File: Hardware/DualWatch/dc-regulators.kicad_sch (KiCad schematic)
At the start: 28 parts, among them Q1 IRLM2803, U16 SN74LV1T34DCK, U2 TPS63030DSK

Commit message: update pcb placing
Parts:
- C? (x2): footprint Capacitor_SMD:C_0402_1005Metric -> Capacitor_SMD:C_0603_1608Metric
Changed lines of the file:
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@@
       (effects (font (size 1.27 1.27)) (justify left))
     )
-    (property "Footprint" "Capacitor_SMD:C_0402_1005Metric" (at 129.2352 104.14 0)
+    (property "Footprint" "Capacitor_SMD:C_0603_1608Metric" (at 129.2352 104.14 0)
       (effects (font (size 1.27 1.27)) hide)
     )
@@
       (effects (font (size 1.27 1.27)) (justify left))
     )
-    (property "Footprint" "Capacitor_SMD:C_0402_1005Metric" (at 128.6002 52.07 0)
+    (property "Footprint" "Capacitor_SMD:C_0603_1608Metric" (at 128.6002 52.07 0)
       (effects (font (size 1.27 1.27)) hide)
     )

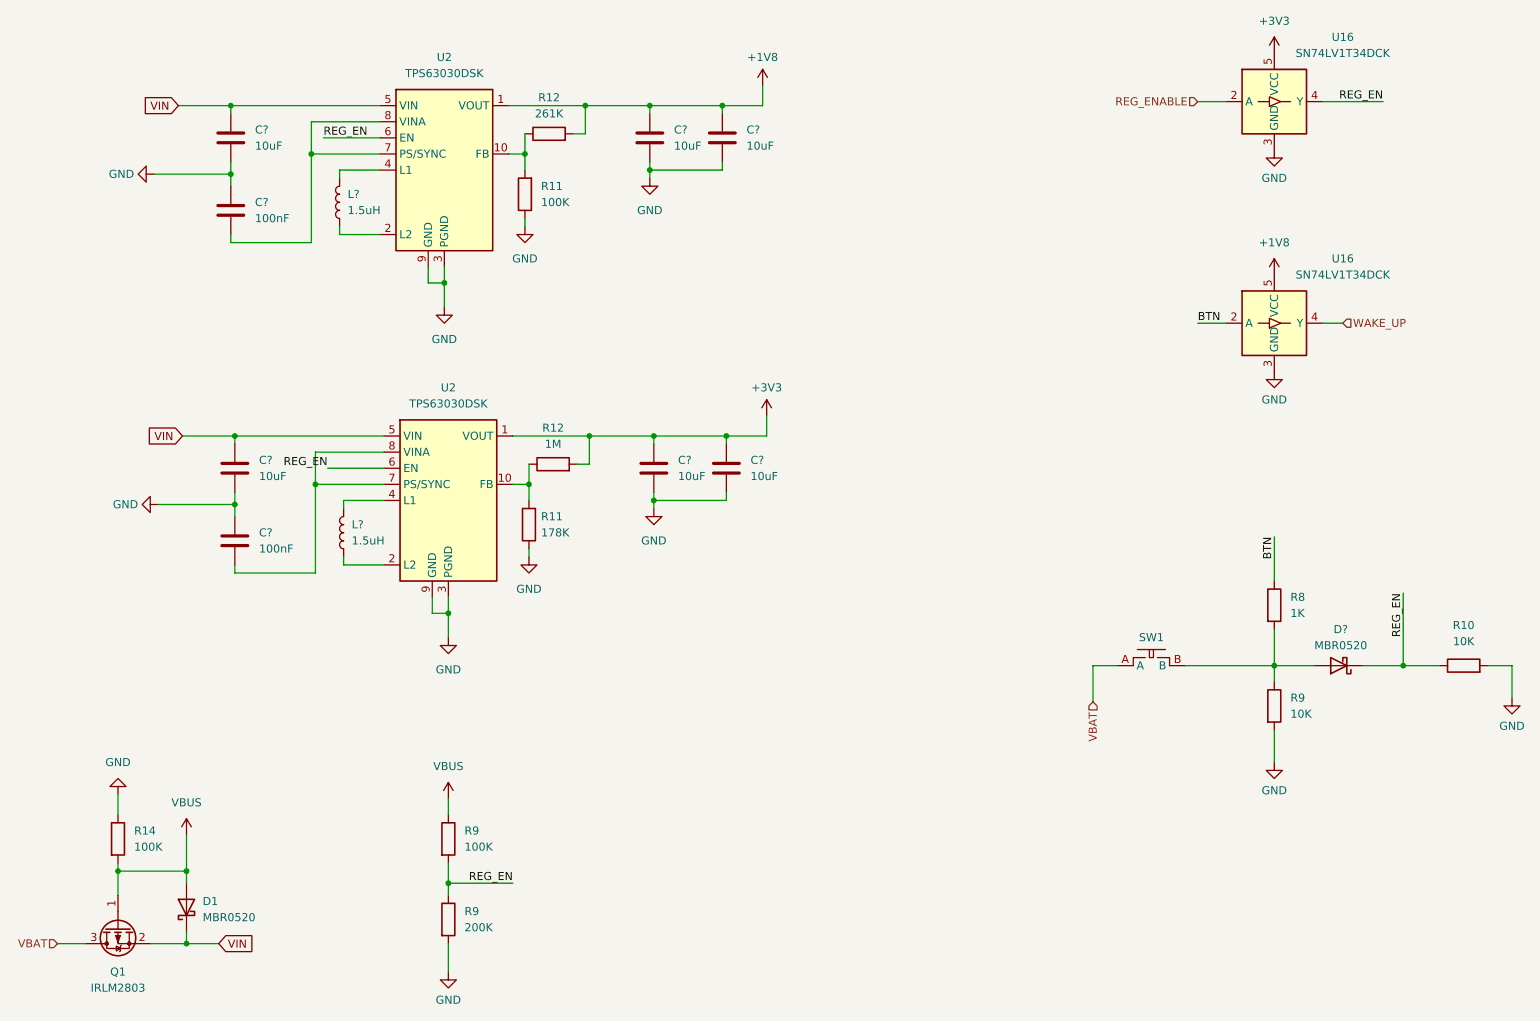
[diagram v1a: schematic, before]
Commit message: update pcb
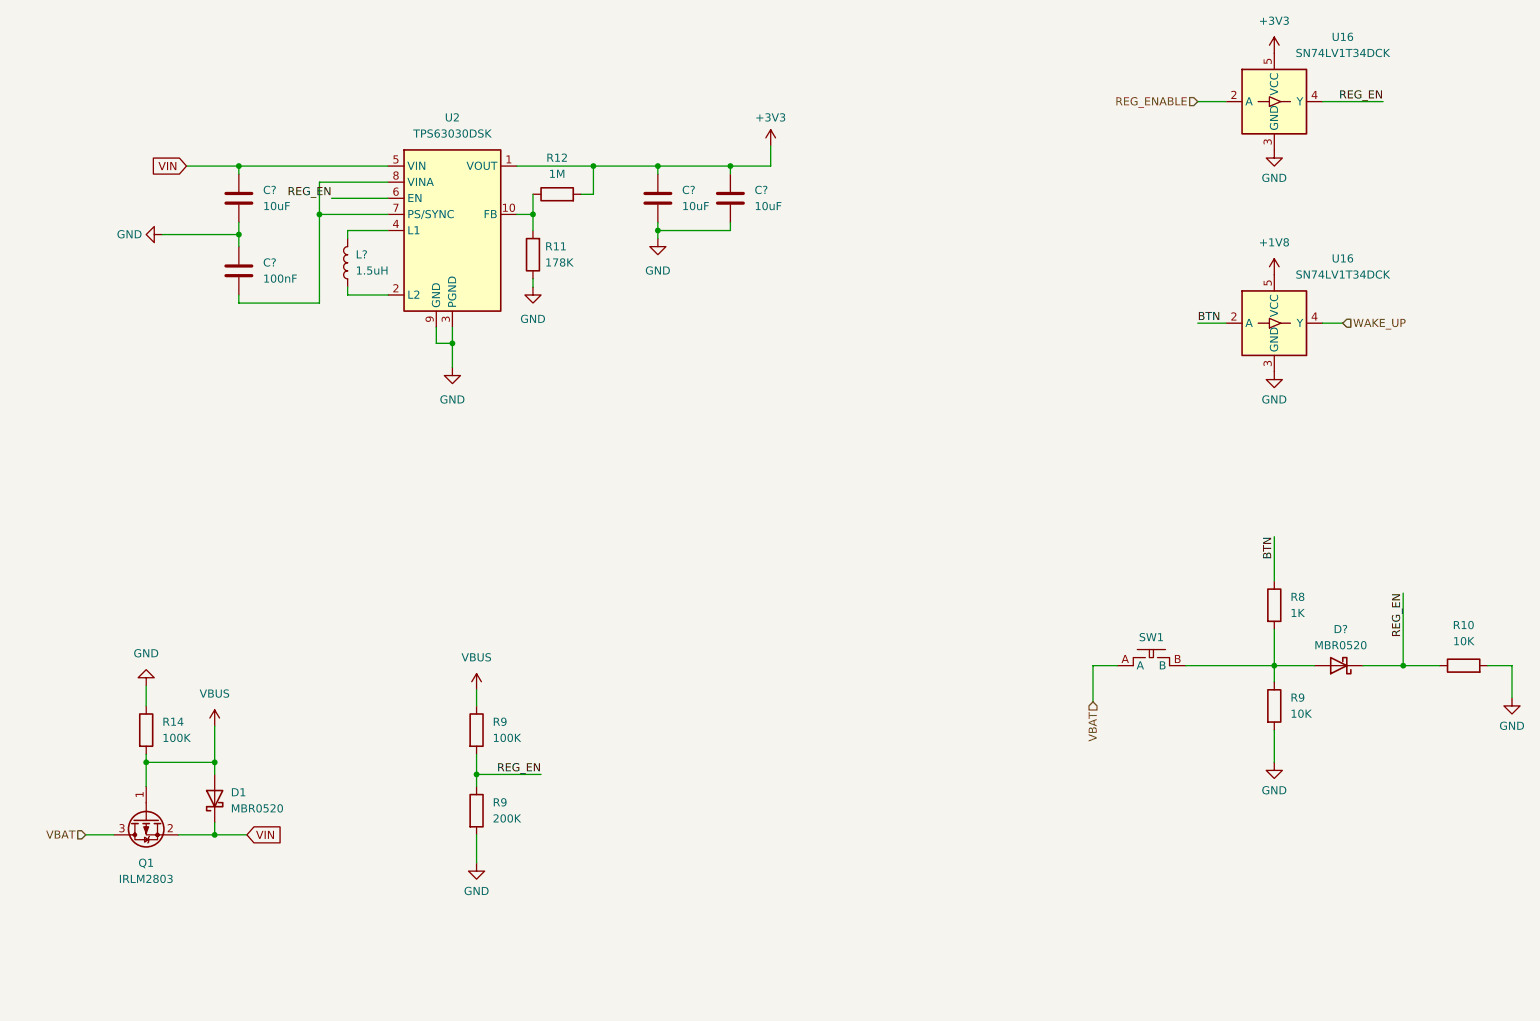
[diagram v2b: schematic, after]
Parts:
- removed C?: 100nF, Capacitor_SMD:C_0402_1005Metric, symbol Device:C
- removed C? (x3): 10uF, Capacitor_SMD:C_0603_1608Metric, symbol Device:C
- removed L?: 1.5uH, Inductor_SMD:L_Coilcraft_XAL4020-XXX, symbol Device:L
- removed R11: 100K, Resistor_SMD:R_0402_1005Metric, symbol Device:R
- removed R12: 261K, Resistor_SMD:R_0402_1005Metric, symbol Device:R
- removed U2: TPS63030DSK, Package_SON:WSON-10-1EP_2.5x2.5mm_P0.5mm_EP1.2x2mm, symbol Regulator_Switching:TPS63030DSK
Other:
- moved on the sheet: C?, D1, L?, Q1, R11, R12, R14, R9, U2

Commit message: Finish Board
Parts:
- L?: footprint Inductor_SMD:L_Coilcraft_XAL4020-XXX -> Inductor_SMD:L_Murata_DFE201610P
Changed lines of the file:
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@@
       (effects (font (size 1.27 1.27)) (justify right))
     )
-    (property "Footprint" "Inductor_SMD:L_Coilcraft_XAL4020-XXX" (at 80.01 67.945 0)
+    (property "Footprint" "Inductor_SMD:L_Murata_DFE201610P" (at 80.01 67.945 0)
       (effects (font (size 1.27 1.27)) hide)
     )
